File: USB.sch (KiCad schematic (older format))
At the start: 0 parts

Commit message: finishing schematic
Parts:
- added C52, C53, C54, C55, C56, C57, C58, C61, C62: 0.1uF, Capacitor_SMD:C_0603_1608Metric, symbol Device:C_Small
- added C59, C60: 22uF, Capacitor_SMD:C_0603_1608Metric, symbol Device:C_Small
- added F1: Fuse_Small, symbol Device:Fuse_Small
- added J2: USB_A, symbol Connector:USB_A
- added J3: USB3_A, symbol Connector:USB3_A
- added L10, L4: 0Ohm, Inductor_SMD:L_0603_1608Metric, symbol pspice:INDUCTOR
- added L3, L5, L6, L9: ACM2012-900, symbol Device:L_Coupled
- added L7, L8: 220Ohm, Inductor_SMD:L_0603_1608Metric, symbol pspice:INDUCTOR
- added U4, U7: TPD4S012DRYR, DRY6, symbol TPD4S012DRYR:TPD4S012DRYR
- added U5: TPS2066DR, D8, symbol TPS2066DR:TPS2066DR
- added U6: TPD4EUSB30, Package_SON:USON-10_2.5x1.0mm_P0.5mm, symbol Power_Protection:TPD4EUSB30
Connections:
- new net: J3.2 (D-), L9.4, U7.2 (D-)
- new net: J3.3 (D+), L9.2, U7.1 (D1+)
- new net: J3.5 (SSRX-), L6.4, U6.5 (D2-)
- new net: J3.6 (SSRX+), L6.2, U6.4 (D2+)
- new net: J3.8 (SSTX-), L5.4, U6.2 (D1-)
- new net: J3.9 (SSTX+), L5.2, U6.1 (D1+)
- new net: J2.2 (D-), L3.2, U4.1 (D1+)
- new net: J2.3 (D+), L3.4, U4.2 (D-)
- new net: C57.2, L5.1
- new net: C58.2, L5.3
- new net: L8.1, U5.6 (OUT2)
- new net: L7.1, U5.7 (OUT1)
- new net: C61.2, L10.2
- new net: C52.2, L4.2
- new net +5VSB: F1.1
- new net +USBVCC: C53.1, C54.1, C55.1, F1.2, U5.2 (IN)
- new net GND: C53.2, C54.2, C55.2, C56.2, C59.2, C60.2, C62.2, J2.4 (GND), J2.5 (Shield), J3.10 (SHIELD), J3.4 (GND), J3.7 (DRAIN), L10.1, L4.1, U4.4 (GND), U5.1 (GND), U6.3 (GND), U6.8 (GND), U7.4 (GND)
- new net USB3_RXN0: L6.3
- new net USB3_RXP0: L6.1
- new net USB3_TXN0: C58.1
- new net USB3_TXP0: C57.1
- new net USB_DN0: L9.3
- new net USB_DN1: L3.3
- new net USB_DP0: L9.1
- new net USB_DP1: L3.1
- new net USB_HOST_EN0: U5.3 (*EN1)
- new net USB_HOST_EN1: U5.4 (*EN2)
- new net USB_HOST_OC0: U5.8 (*OC1)
- new net USB_HOST_OC1: U5.5 (*OC2)
- new net VBUS1: C60.1, C61.1, C62.1, J3.1 (VBUS), L7.2, U7.6 (VBUS)
- new net VBUS2: C52.1, C56.1, C59.1, J2.1 (VBUS), L8.2, U4.6 (VBUS)

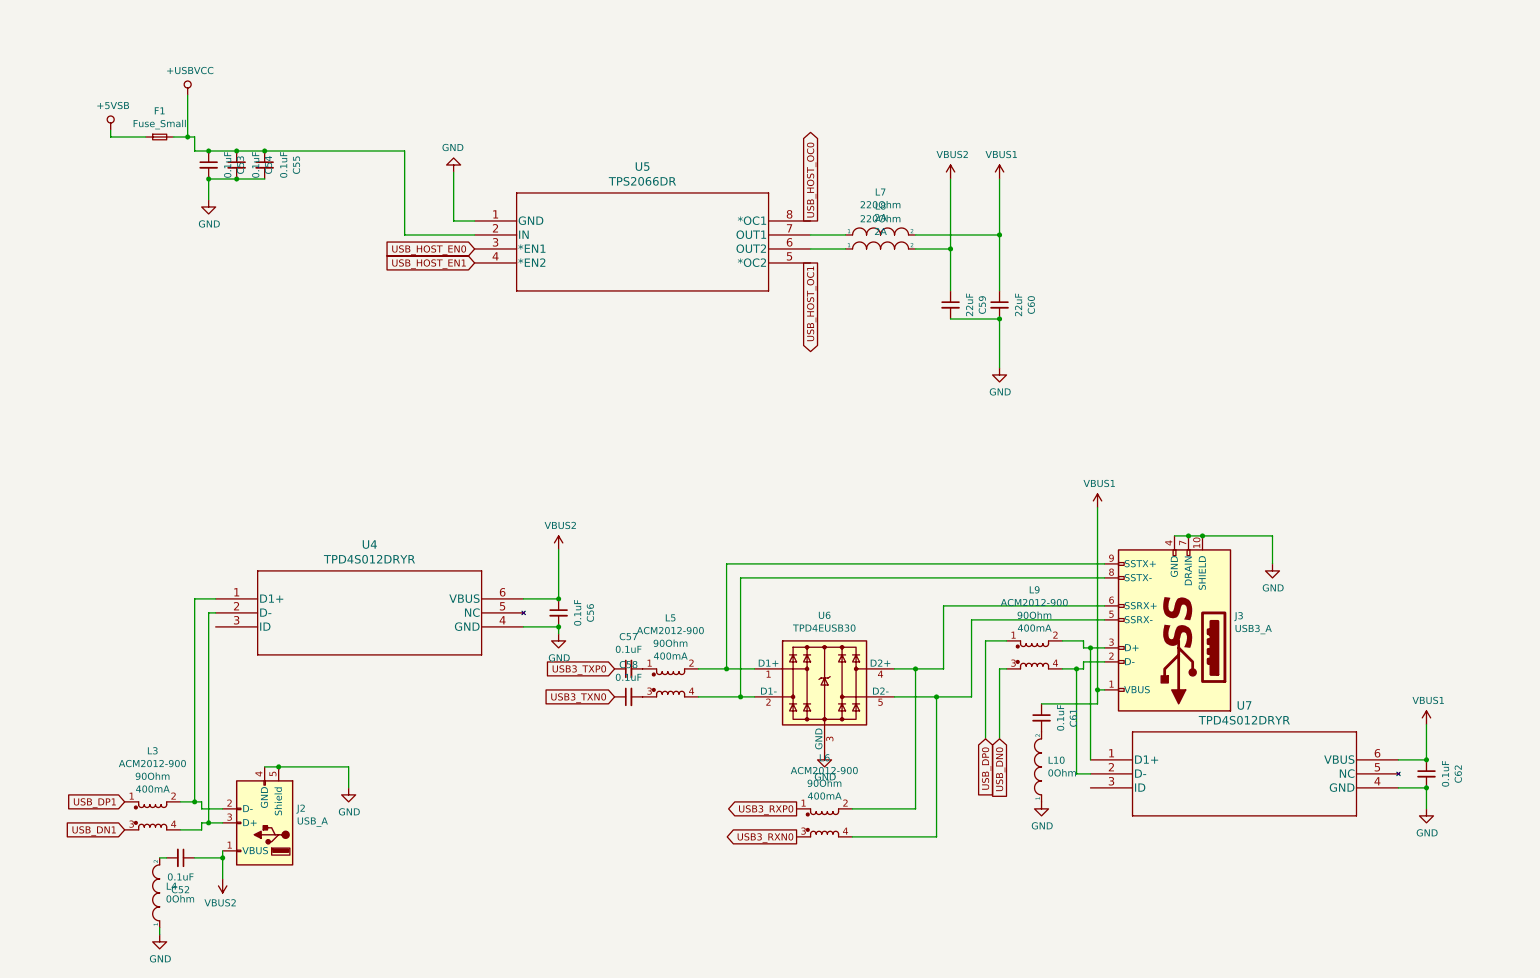
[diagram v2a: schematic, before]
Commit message: finished fixes
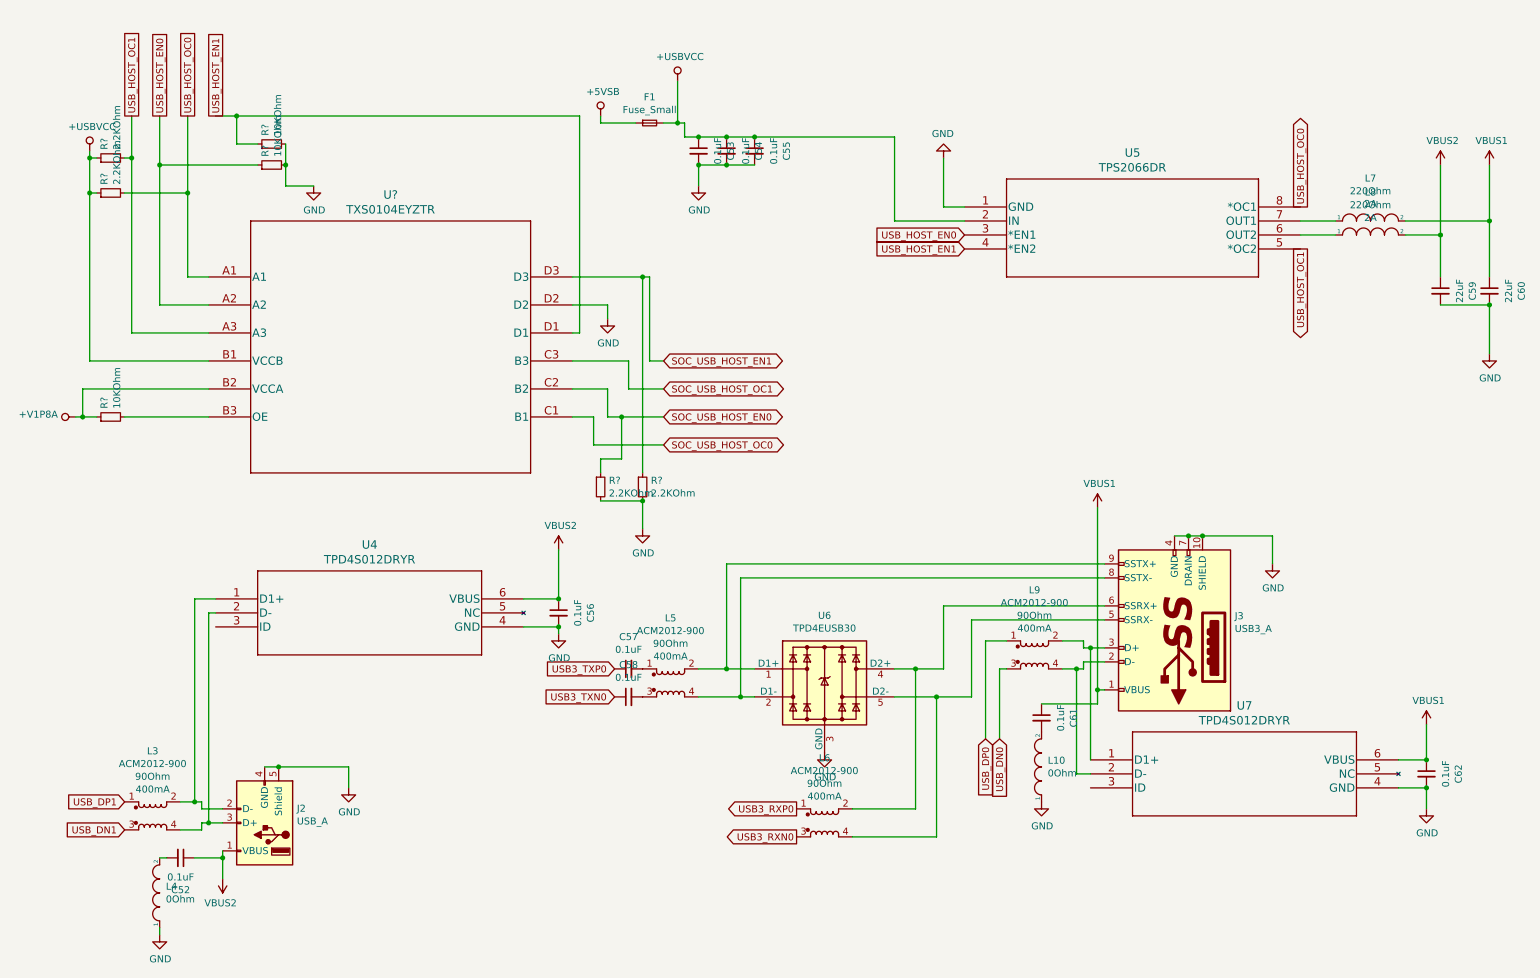
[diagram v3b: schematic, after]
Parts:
- added R? (x3): 10KOhm, Resistor_SMD:R_0603_1608Metric, symbol Device:R_Small
- added R? (x4): 2.2KOhm, Resistor_SMD:R_0603_1608Metric, symbol Device:R_Small
- added U?: TXS0104EYZTR, YZT12, symbol TXS0104EYZTR:TXS0104EYZTR
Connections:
- net +USBVCC: now also R?.1, R?.1, U?.B1 (VCCB)
- net GND: now also R?.2, R?.2, R?.2, R?.2, U?.D2
- net USB_HOST_EN0: now also R?.1, U?.A2
- net USB_HOST_EN1: now also R?.1, U?.D1
- net USB_HOST_OC0: now also R?.2, U?.A1
- net USB_HOST_OC1: now also R?.2, U?.A3
- new net: R?.2, U?.B3 (OE)
- new net +V1P8A: R?.1, U?.B2 (VCCA)
- new net SOC_USB_HOST_EN0: R?.1, U?.C2 (B2)
- new net SOC_USB_HOST_EN1: R?.1, U?.D3
- new net SOC_USB_HOST_OC0: U?.C1 (B1)
- new net SOC_USB_HOST_OC1: U?.C3 (B3)
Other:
- moved on the sheet: C53, C54, C55, C59, C60, F1, L7, L8, U5
